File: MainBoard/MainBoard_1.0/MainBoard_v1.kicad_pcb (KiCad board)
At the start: 2 copper layers, 122 x 85.6 mm, 173 parts, among them J1 ILG, J10 SH, J11 SH, J12 SH, J13 FFC, J14 SH, J2 SH, J3 SH, J4 PA, J5 Micro_SD_Card_Det_Hirose_DM3AT, J6 SH, J7 ENC, J8 ENC, J9 PA, Q1 AON7400B, Q10 IRLML6344, Q2 AON7400B, Q3 AON7400B, Q4 AON7400B, Q5 AON7400B, Q6 AON7400B, Q7 2N7002K, Q8 AON7400B, Q9 AON7400B, SW1 SKRPACE010, SW2 SSSS213202, SW3 FR01SC16P-S, SW4 SKRHAAE010, U1 SI7469DP-T1-GE3, U10 DRV8701E, U11 MMC5983MA, U2 LT1963A-TSSOP, U3 TPS62143, U4 ECS-2520S33, U5 INA260, U6 DRV8701E, U7 ICM20648, U8 STM32F469VG, U9 INA260

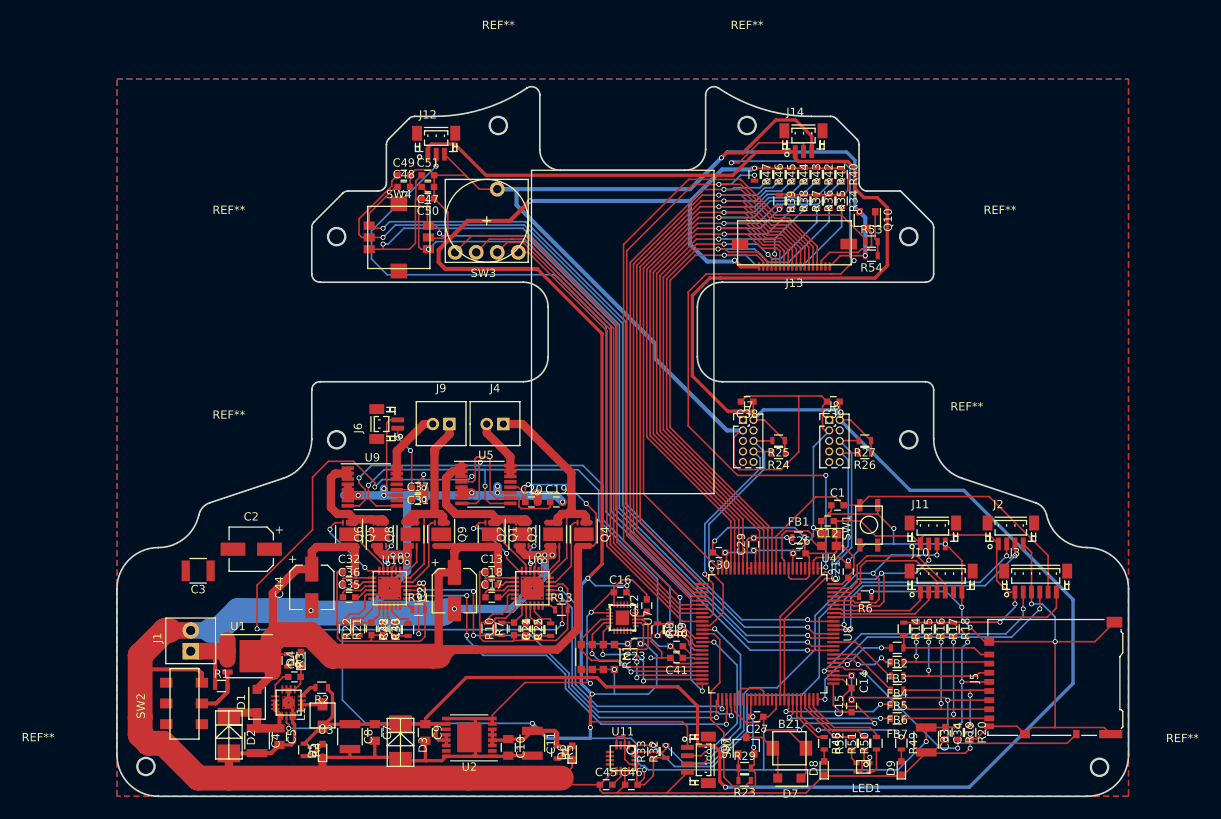
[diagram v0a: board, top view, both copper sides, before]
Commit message: update edge
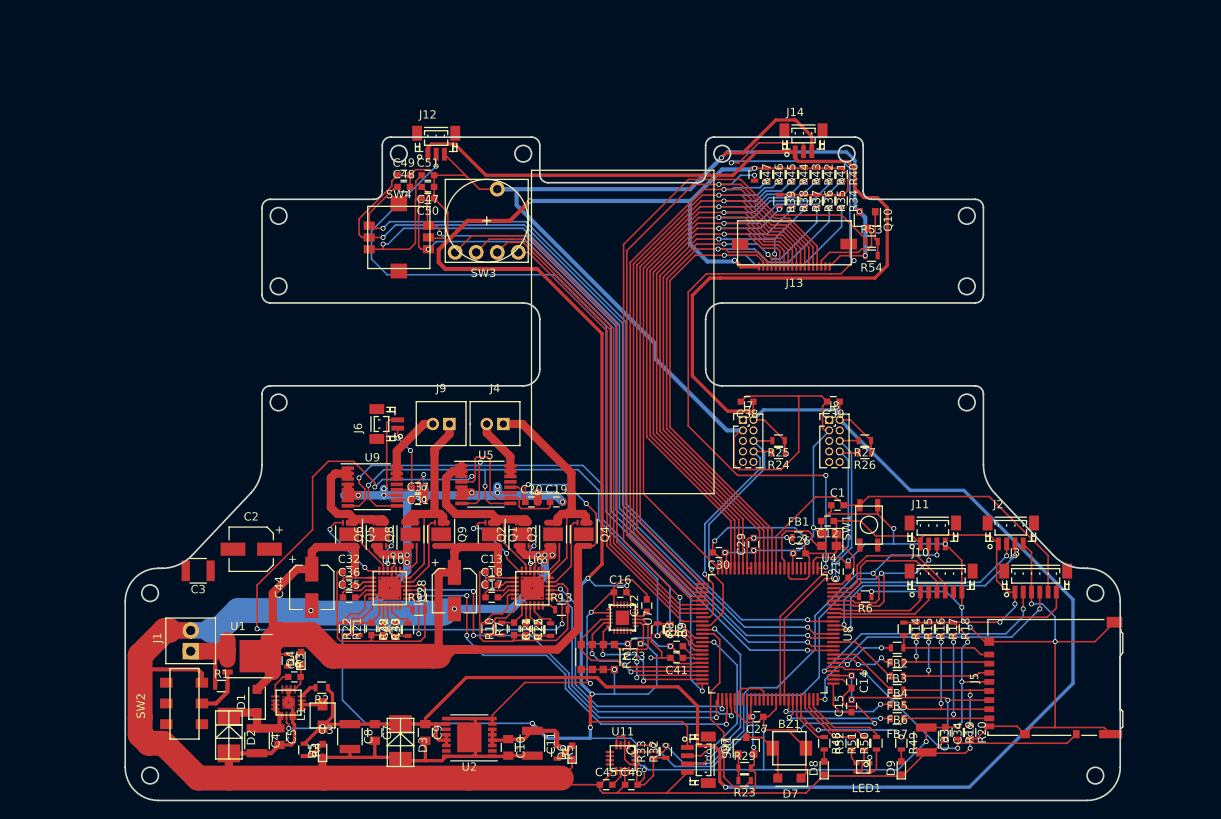
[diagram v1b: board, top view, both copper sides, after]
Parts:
- removed REF** (x8): MountingHole_2.2mm_M2, Mounting_Holes:MountingHole_2.2mm_M2
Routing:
- removed copper zone on B.Cu, net GND
- removed copper zone on F.Cu, net GND
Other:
- board size 122 x 85.6 mm -> 120 x 80 mm
